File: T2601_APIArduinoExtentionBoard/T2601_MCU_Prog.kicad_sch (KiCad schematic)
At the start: 6 parts, among them J28 Conn_02x03_Counter_Clockwise

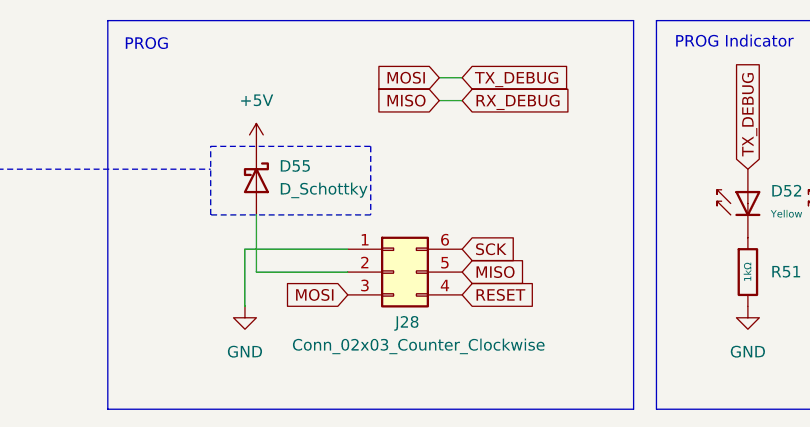
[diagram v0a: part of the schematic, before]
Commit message: Reroutage en cours 2
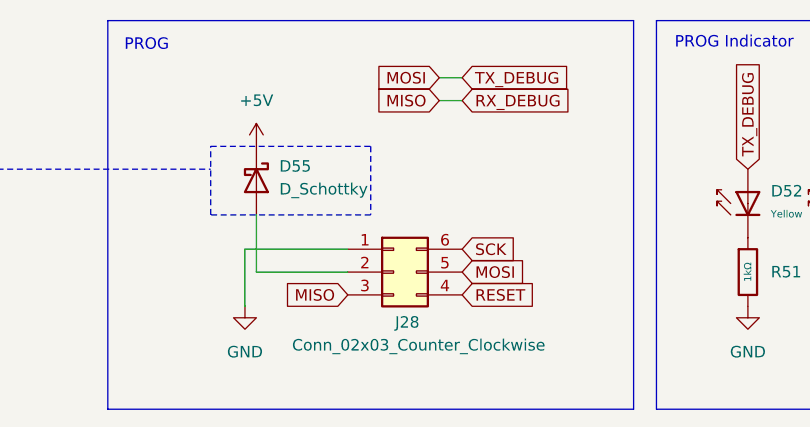
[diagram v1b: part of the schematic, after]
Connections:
- net MISO: now also J28.3 (Pin_3); no longer J28.5 (Pin_5)
- net MOSI: now also J28.5 (Pin_5); no longer J28.3 (Pin_3)
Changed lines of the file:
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@@
 	(global_label "MISO"
 		(shape input)
-		(at 142.24 95.25 0)
+		(at 129.54 97.79 180)
 		(fields_autoplaced yes)
 		(effects
@@
 				(size 1.27 1.27)
 			)
-			(justify left)
+			(justify right)
 		)
 		(property "Intersheetrefs" "${INTERSHEET_REFS}"
-			(at 149.8214 95.25 0)
+			(at 122.3341 97.79 0)
 			(hide yes)
 			(show_name no)
@@
 					(size 1.27 1.27)
 				)
-				(justify left)
+				(justify right)
 			)
 		)
@@
 	(global_label "MOSI"
 		(shape input)
-		(at 129.54 97.79 180)
+		(at 142.24 95.25 0)
 		(fields_autoplaced yes)
 		(effects
@@
 				(size 1.27 1.27)
 			)
-			(justify right)
+			(justify left)
 		)
 		(property "Intersheetrefs" "${INTERSHEET_REFS}"
-			(at 121.9586 97.79 0)
+			(at 149.4459 95.25 0)
 			(hide yes)
 			(show_name no)
@@
 					(size 1.27 1.27)
 				)
-				(justify right)
+				(justify left)
 			)
 		)
